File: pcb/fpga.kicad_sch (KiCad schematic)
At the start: 41 parts, among them J2 Conn_01x06, U1 ICE40HX1K-VQ100, U2 W25Q16JVZPIQ, U3 AP2127N-1.2, Y1 AMPMAFB-25.0000T

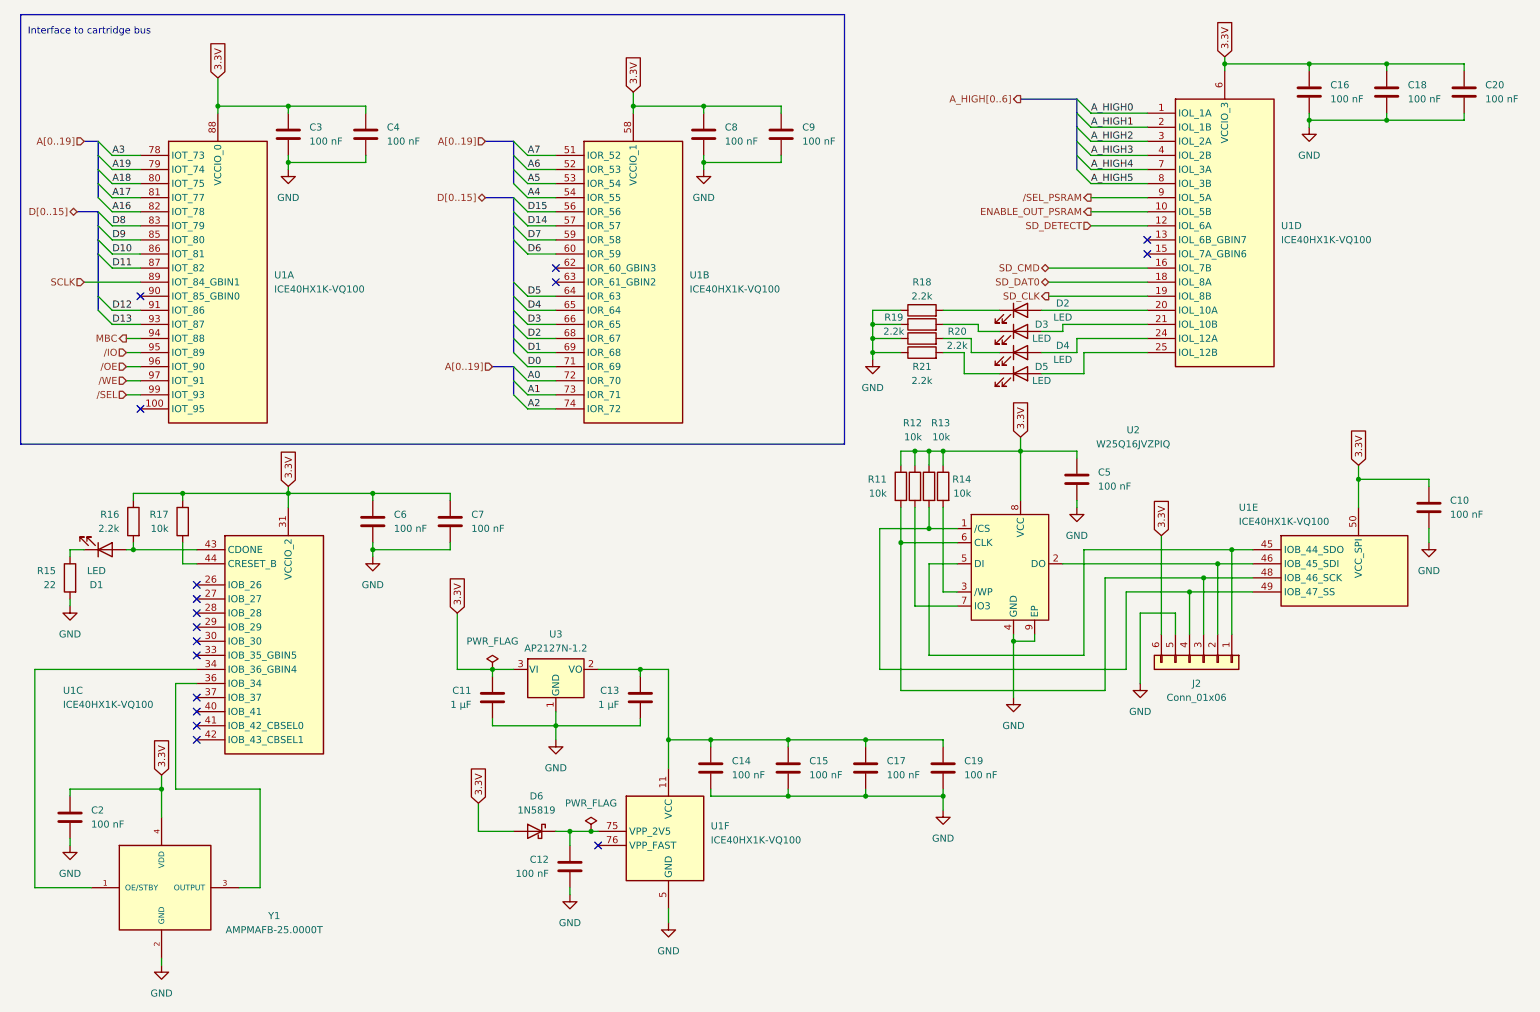
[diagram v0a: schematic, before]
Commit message: second pcb iteration
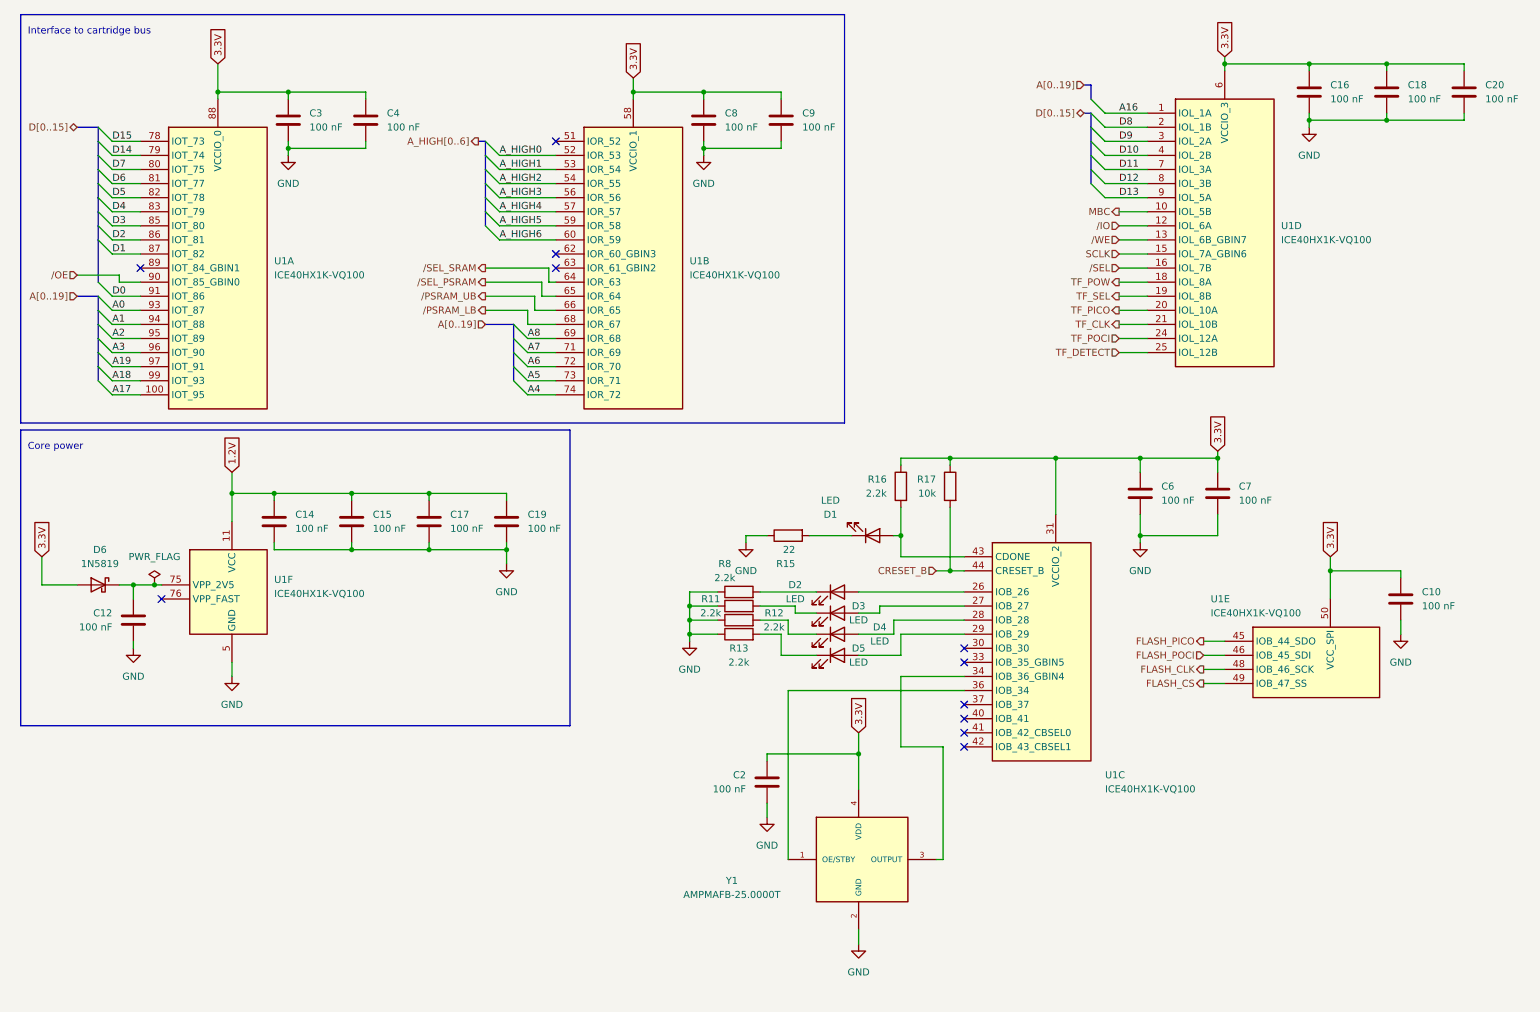
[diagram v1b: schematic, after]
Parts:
- removed C11, C13: 1 μF, Capacitor_SMD:C_0603_1608Metric, symbol Device:C
- removed C5: 100 nF, Capacitor_SMD:C_0603_1608Metric, symbol Device:C
- removed J2: Conn_01x06, Connector_PinSocket_1.27mm:PinSocket_1x06_P1.27mm_Vertical, symbol Connector_Generic:Conn_01x06
- removed R14: 10k, Resistor_SMD:R_0603_1608Metric, symbol Device:R
- removed R18, R19, R20, R21: 2.2k, Resistor_SMD:R_0603_1608Metric, symbol Device:R
- removed U2: W25Q16JVZPIQ, snapeda:SON127P500X600X80-9N, symbol nileswan:W25Q16JVZPIQ
- removed U3: AP2127N-1.2, Package_TO_SOT_SMD:SOT-23, symbol Regulator_Linear:AP2127N-1.2
- added R8: 2.2k, Resistor_SMD:R_0402_1005Metric, symbol Device:R
- C10, C12, C14, C15, C16, C17, C18, C19, C2, C20, C3, C4, C6, C7, C8, C9: footprint Capacitor_SMD:C_0603_1608Metric -> Capacitor_SMD:C_0402_1005Metric
- D1, D2, D3, D4, D5: footprint LED_SMD:LED_0603_1608Metric -> LED_SMD:LED_0402_1005Metric
- R11, R12, R13: value 10k -> 2.2k; footprint Resistor_SMD:R_0603_1608Metric -> Resistor_SMD:R_0402_1005Metric
- R15, R16, R17: footprint Resistor_SMD:R_0603_1608Metric -> Resistor_SMD:R_0402_1005Metric
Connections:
- net ENABLE_OUT_PSRAM is gone; now on net MBC: U1.10 (IOL_5B)
- net SD_CMD is gone; now on net /SEL: U1.16 (IOL_7B)
- net SD_DETECT is gone; now on net /IO: U1.12 (IOL_6A)
- net 3.3V: no longer R11.1, R12.1, R13.1
- net A0: now also U1.93 (IOT_87); no longer U1.72 (IOR_70)
- net A1: now also U1.94 (IOT_88); no longer U1.73 (IOR_71)
- net A16: now also U1.1 (IOL_1A); no longer U1.82 (IOT_78)
- net A17: now also U1.100 (IOT_95); no longer U1.81 (IOT_77)
- net A18: now also U1.99 (IOT_93); no longer U1.80 (IOT_75)
- net A19: now also U1.97 (IOT_91); no longer U1.79 (IOT_74)
- net A2: now also U1.95 (IOT_89); no longer U1.74 (IOR_72)
- net A3: now also U1.96 (IOT_90); no longer U1.78 (IOT_73)
- net A4: now also U1.74 (IOR_72); no longer U1.54 (IOR_55)
- net A5: now also U1.73 (IOR_71); no longer U1.53 (IOR_54)
- net A6: now also U1.72 (IOR_70); no longer U1.52 (IOR_53)
- net A7: now also U1.71 (IOR_69); no longer U1.51 (IOR_52)
- net A_HIGH0: now also U1.52 (IOR_53); no longer U1.1 (IOL_1A)
- net A_HIGH1: now also U1.53 (IOR_54); no longer U1.2 (IOL_1B)
- net A_HIGH2: now also U1.54 (IOR_55); no longer U1.3 (IOL_2A)
- net A_HIGH3: now also U1.56 (IOR_56); no longer U1.4 (IOL_2B)
- net A_HIGH4: now also U1.57 (IOR_57); no longer U1.7 (IOL_3A)
- net A_HIGH5: now also U1.59 (IOR_58); no longer U1.8 (IOL_3B)
- net D0: now also U1.91 (IOT_86); no longer U1.71 (IOR_69)
- net D1: now also U1.87 (IOT_82); no longer U1.69 (IOR_68)
- net D10: now also U1.4 (IOL_2B); no longer U1.86 (IOT_81)
- net D11: now also U1.7 (IOL_3A); no longer U1.87 (IOT_82)
- net D12: now also U1.8 (IOL_3B); no longer U1.91 (IOT_86)
- net D13: now also U1.9 (IOL_5A); no longer U1.93 (IOT_87)
- net D14: now also U1.79 (IOT_74); no longer U1.57 (IOR_57)
- net D15: now also U1.78 (IOT_73); no longer U1.56 (IOR_56)
- net D2: now also U1.86 (IOT_81); no longer U1.68 (IOR_67)
- net D3: now also U1.85 (IOT_80); no longer U1.66 (IOR_65)
- net D4: now also U1.83 (IOT_79); no longer U1.65 (IOR_64)
- net D5: now also U1.82 (IOT_78); no longer U1.64 (IOR_63)
- net D6: now also U1.81 (IOT_77); no longer U1.60 (IOR_59)
- net D7: now also U1.80 (IOT_75); no longer U1.59 (IOR_58)
- net D8: now also U1.2 (IOL_1B); no longer U1.83 (IOT_79)
- net D9: now also U1.3 (IOL_2A); no longer U1.85 (IOT_80)
- net GND: now also R11.1, R12.1, R13.1, R15.1, R8.1; no longer R15.2
- net MBC: no longer U1.94 (IOT_88)
- net SCLK: now also U1.15 (IOL_7A_GBIN6); no longer U1.89 (IOT_84_GBIN1)
- net /IO: no longer U1.95 (IOT_89)
- net /OE: now also U1.90 (IOT_85_GBIN0); no longer U1.96 (IOT_90)
- net /SEL: no longer U1.99 (IOT_93)
- net /SEL_PSRAM: now also U1.65 (IOR_64); no longer U1.9 (IOL_5A)
- net /WE: now also U1.13 (IOL_6B_GBIN7); no longer U1.97 (IOT_91)
- net at D4.1 (K): now also R12.2
- net at D4.2 (A): now also U1.28 (IOB_28); no longer U1.24 (IOL_12A)
- net at D5.1 (K): now also R13.2
- net at D5.2 (A): now also U1.29 (IOB_29); no longer U1.25 (IOL_12B)
- net at D3.1 (K): now also R11.2
- net FLASH_PICO: now reaches U1.45 (IOB_44_SDO)
- net FLASH_POCI: now reaches U1.46 (IOB_45_SDI)
- net FLASH_CLK: now reaches U1.48 (IOB_46_SCK)
- net FLASH_CLK: no longer R11.2
- net FLASH_CS: now reaches U1.49 (IOB_47_SS)
- net FLASH_CS: no longer R13.2
- net at D2.2 (A): now also U1.26 (IOB_26); no longer U1.20 (IOL_10A)
- net at D3.2 (A): now also U1.27 (IOB_27); no longer U1.21 (IOL_10B)
- net at D2.1 (K): now also R8.2
- net 1.2V: now reaches C14.1, C15.1, C17.1, C19.1, U1.11 (VCC), U1.35 (VCC), U1.61 (VCC), U1.77 (VCC)
- net at U1.34 (IOB_36_GBIN4): now also Y1.3 (OUTPUT); no longer Y1.1 (OE/STBY)
- net at U1.36 (IOB_34): now also Y1.1 (OE/STBY); no longer Y1.3 (OUTPUT)
- net CRESET_B: now reaches R17.2, U1.44 (CRESET_B)
- net at D1.1 (K): now also R15.2; no longer R15.1
- net SD_CLK renamed TF_SEL
- net SD_DAT0 renamed TF_POW
- new net A8: U1.69 (IOR_68)
- new net A_HIGH6: U1.60 (IOR_59)
- new net TF_CLK: U1.21 (IOL_10B)
- new net TF_DETECT: U1.25 (IOL_12B)
- new net TF_PICO: U1.20 (IOL_10A)
- new net TF_POCI: U1.24 (IOL_12A)
- new net /PSRAM_LB: U1.68 (IOR_67)
- new net /PSRAM_UB: U1.66 (IOR_65)
- new net /SEL_SRAM: U1.64 (IOR_63)
- no-connect marks 17 -> 11
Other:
- note added: "Core power"
- moved on the sheet: C10, C12, C14, C15, C17, C19, C2, C3, C4, C6, C7, C8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
